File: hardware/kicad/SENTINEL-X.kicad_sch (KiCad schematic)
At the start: 7 parts, among them U1 NodeMCU_ESP8266

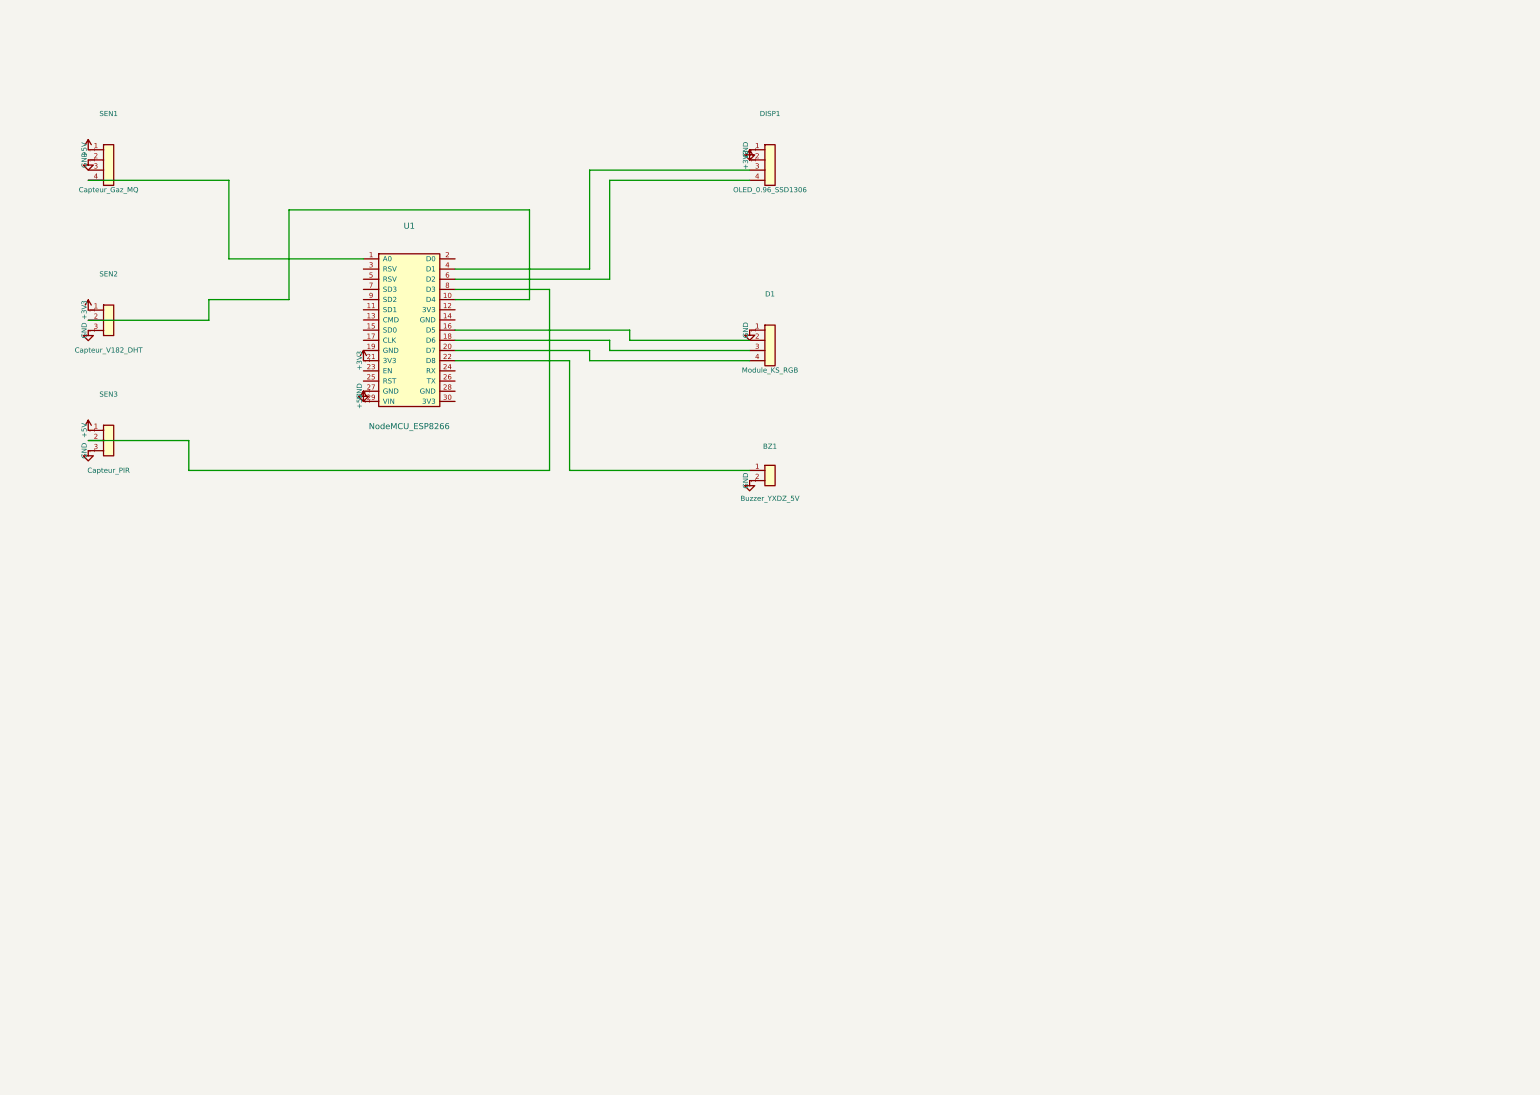
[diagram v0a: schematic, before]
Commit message: fix
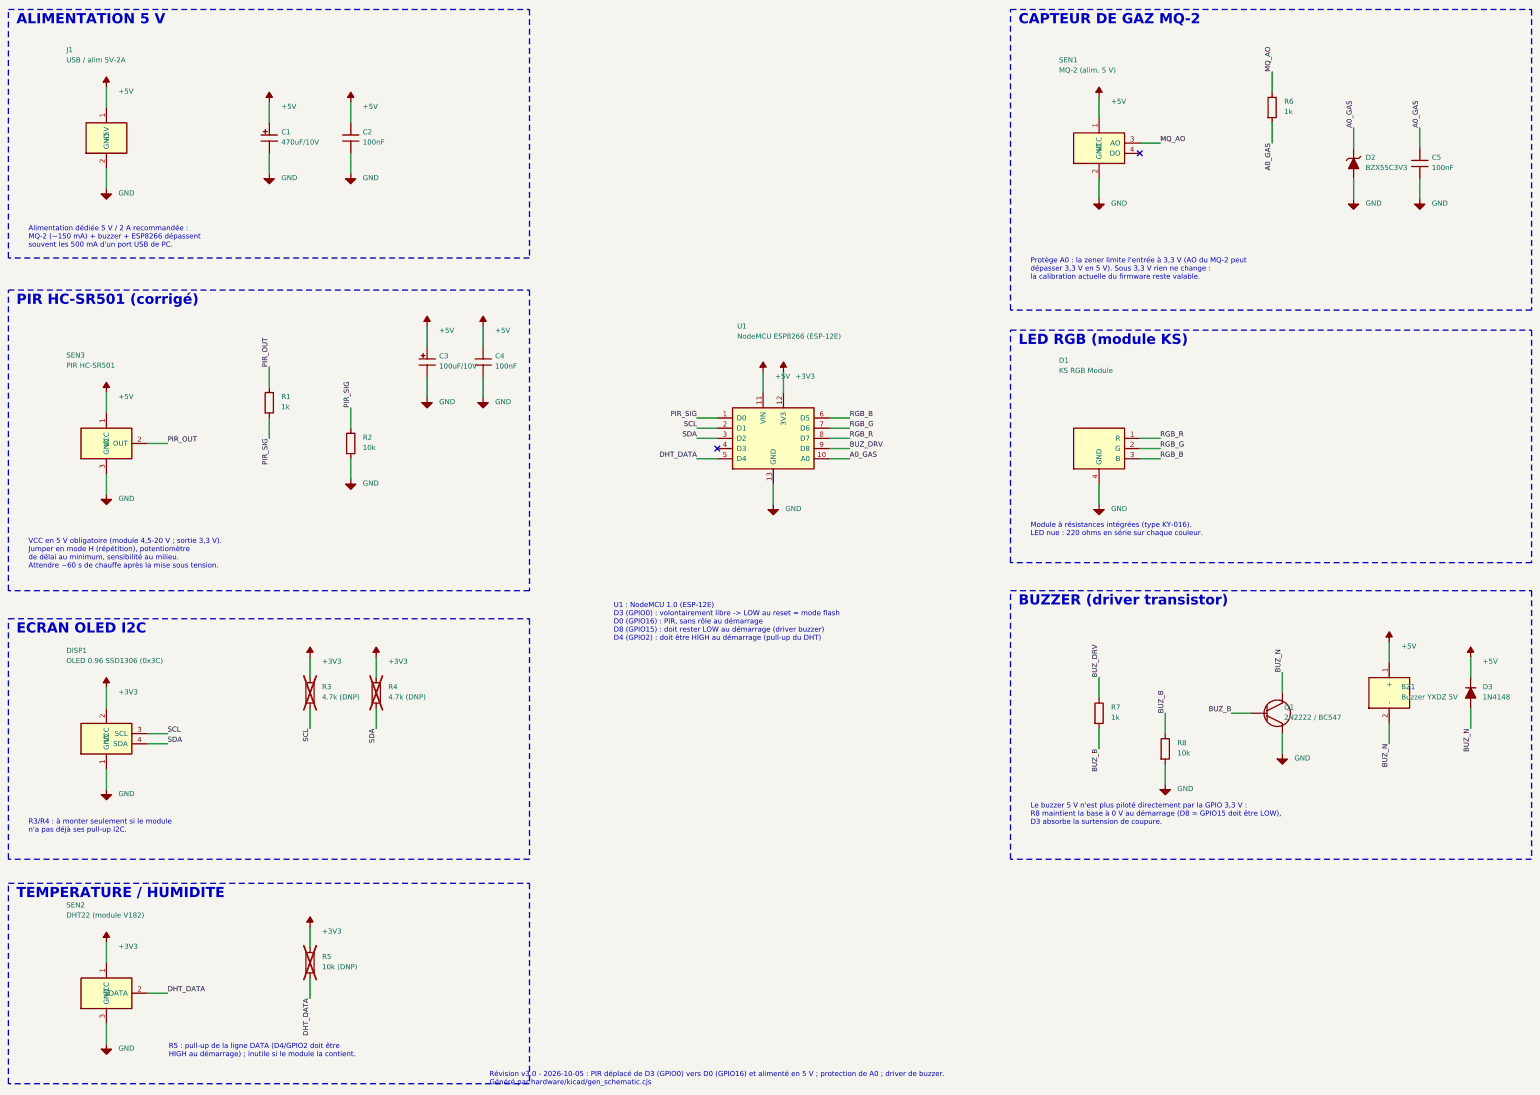
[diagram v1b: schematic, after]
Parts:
- removed BZ1: Buzzer_YXDZ_5V, symbol Connector_Generic:Conn_01x02
- removed D1: Module_KS_RGB, symbol Connector_Generic:Conn_01x04
- removed DISP1: OLED_0.96_SSD1306, symbol Connector_Generic:Conn_01x04
- removed SEN1: Capteur_Gaz_MQ, symbol Connector_Generic:Conn_01x04
- removed SEN2: Capteur_V182_DHT, symbol Connector_Generic:Conn_01x03
- removed SEN3: Capteur_PIR, symbol Connector_Generic:Conn_01x03
- removed U1: NodeMCU_ESP8266, symbol Connector_Generic:Conn_02x15_Odd_Even
- added BZ1: Buzzer YXDZ 5V, symbol SENTINEL:Buzzer_5V
- added C1: 470uF/10V, symbol SENTINEL:C_Polarized
- added C2, C4, C5: 100nF, symbol SENTINEL:C
- added C3: 100uF/10V, symbol SENTINEL:C_Polarized
- added D1: KS RGB Module, symbol SENTINEL:KS_RGB_Module
- added D2: BZX55C3V3, symbol SENTINEL:D_Zener
- added D3: 1N4148, symbol SENTINEL:D
- added DISP1: OLED 0.96 SSD1306 (0x3C), symbol SENTINEL:OLED_SSD1306_I2C
- added J1: USB / alim 5V-2A, symbol SENTINEL:Alim_5V
- added Q1: 2N2222 / BC547, symbol SENTINEL:Q_NPN
- added R1, R6, R7: 1k, symbol SENTINEL:R
- added R2, R8: 10k, symbol SENTINEL:R
- added R3, R4: 4.7k (DNP), symbol SENTINEL:R
- added R5: 10k (DNP), symbol SENTINEL:R
- added SEN1: MQ-2 (alim. 5 V), symbol SENTINEL:MQ-2_Module
- added SEN2: DHT22 (module V182), symbol SENTINEL:DHT22_V182
- added SEN3: PIR HC-SR501, symbol SENTINEL:PIR_HC-SR501
- added U1: NodeMCU ESP8266 (ESP-12E), symbol SENTINEL:NodeMCU_ESP8266
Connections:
- net +3V3: now also DISP1.2 (VCC), R3.1, R4.1, R5.1, SEN2.1 (VCC), U1.12 (3V3)
- net +5V: now also BZ1.1 (+), C1.1, C2.1, C3.1, C4.1, D3.1 (K), J1.1 (+5V), SEN1.1 (VCC), SEN3.1 (VCC), U1.11 (VIN)
- net GND: now also C1.2, C2.2, C3.2, C4.2, C5.2, D1.4 (GND), D2.2 (A), DISP1.1 (GND), J1.2 (GND), Q1.1 (E), R2.2, R8.2, SEN1.2 (GND), SEN2.3 (GND), SEN3.3 (GND), U1.13 (GND)
- new net A0_GAS: C5.1, D2.1 (K), R6.2, U1.10 (A0)
- new net BUZ_B: Q1.2 (B), R7.2, R8.1
- new net BUZ_DRV: R7.1, U1.9 (D8)
- new net BUZ_N: BZ1.2 (-), D3.2 (A), Q1.3 (C)
- new net DHT_DATA: R5.2, SEN2.2 (DATA), U1.5 (D4)
- new net MQ_AO: R6.1, SEN1.3 (AO)
- new net PIR_OUT: R1.1, SEN3.2 (OUT)
- new net PIR_SIG: R1.2, R2.1, U1.1 (D0)
- new net RGB_B: D1.3 (B), U1.6 (D5)
- new net RGB_G: D1.2 (G), U1.7 (D6)
- new net RGB_R: D1.1 (R), U1.8 (D7)
- new net SCL: DISP1.3 (SCL), R3.2, U1.2 (D1)
- new net SDA: DISP1.4 (SDA), R4.2, U1.3 (D2)
- no-connect marks 0 -> 2
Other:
- note added: "ALIMENTATION 5 V"
- note added: "Alimentation dédiée 5 V / 2 A recommandée : MQ-2 (~150 mA) + buzzer + ESP8266 dépassent souvent les 500 mA d'un port USB de PC."
- note added: "BUZZER (driver transistor)"
- note added: "CAPTEUR DE GAZ MQ-2"
- note added: "ECRAN OLED I2C"
- note added: "LED RGB (module KS)"
- note added: "Le buzzer 5 V n'est plus piloté directement par la GPIO 3,3 V : R8 maintient la base à 0 V au démarrage (D8 = GPIO15 doit être LOW), D3 absorbe la surtension de coupure."
- note added: "Module à résistances intégrées (type KY-016). LED nue : 220 ohms en série sur chaque couleur."
- note added: "PIR HC-SR501 (corrigé)"
- note added: "Protège A0 : la zener limite l'entrée à 3,3 V (AO du MQ-2 peut dépasser 3,3 V en 5 V). Sous 3,3 V rien ne change : la calibration actuelle du firmware reste valable."
- note added: "R3/R4 : à monter seulement si le module n'a pas déjà ses pull-up I2C."
- note added: "R5 : pull-up de la ligne DATA (D4/GPIO2 doit être HIGH au démarrage) ; inutile si le module la contient."
- note added: "Révision v3.0 - 2026-10-05 : PIR déplacé de D3 (GPIO0) vers D0 (GPIO16) et alimenté en 5 V ; protection de A0 ; driver de buzzer. Généré par hardware/kicad/gen_schematic.cjs"
- note added: "TEMPERATURE / HUMIDITE"
- note added: "U1 : NodeMCU 1.0 (ESP-12E) D3 (GPIO0) : volontairement libre -> LOW au reset = mode flash D0 (GPIO16) : PIR, sans rôle au démarrage D8 (GPIO15) : doit rester LOW au démarrage (driver buzzer) D4 (GPIO2) : doit être HIGH au démarrage (pull-up du DHT)"
- note added: "VCC en 5 V obligatoire (module 4,5-20 V ; sortie 3,3 V). Jumper en mode H (répétition), potentiomètre de délai au minimum, sensibilité au milieu. Attendre ~60 s de chauffe après la mise sous tension."
